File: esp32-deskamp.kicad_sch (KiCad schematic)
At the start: 29 parts, among them J1 INPUT 00, J10 ADDITIONAL GPIO, J2 INPUT 01, J3 MUTE, J4 SLEEP, J5 PRE OUT, J6 LFE OUT, J7 INPUT SELECT, J8 MOTOR, J9 12V IN, K1 INPUT 00, K2 INPUT 01, K3 AMP MUTE, K4 AMP SLEEP, U1 ESP32 D1 MINI, U2 TSR 1-2433, U3 L9110, U4 ULN2003A

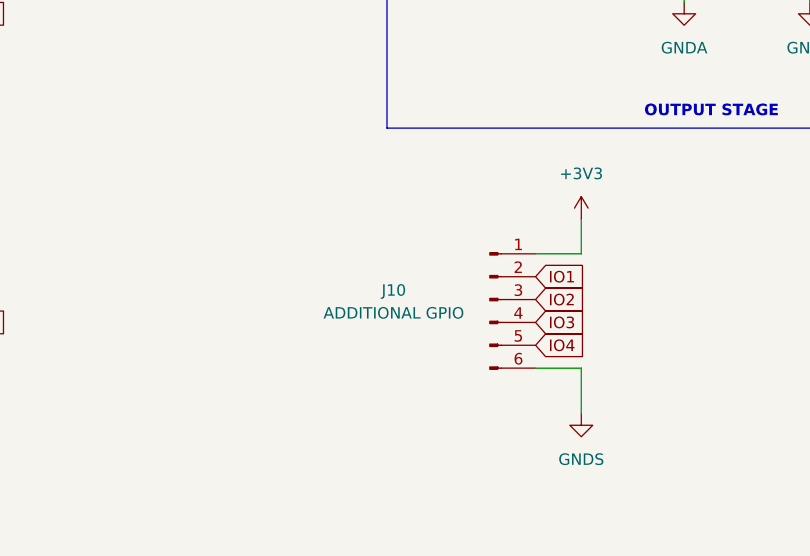
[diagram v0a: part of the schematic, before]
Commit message: Move cap
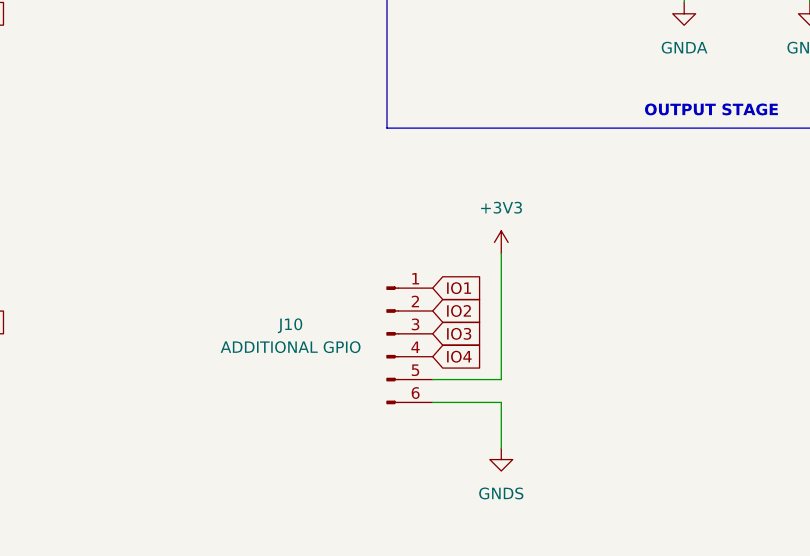
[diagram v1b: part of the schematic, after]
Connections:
- net +3V3: now also J10.5 (Pin_5); no longer J10.1 (Pin_1)
- net IO1: now also J10.1 (Pin_1); no longer J10.2 (Pin_2)
- net IO2: now also J10.2 (Pin_2); no longer J10.3 (Pin_3)
- net IO3: now also J10.3 (Pin_3); no longer J10.4 (Pin_4)
- net IO4: now also J10.4 (Pin_4); no longer J10.5 (Pin_5)
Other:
- moved on the sheet: J10
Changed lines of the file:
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@@
 	(wire
 		(pts
+			(xy 148.59 173.99) (xy 156.21 173.99)
+		)
+		(stroke
+			(width 0)
+			(type default)
+		)
+	)
+	(wire
+		(pts
 			(xy 46.99 31.75) (xy 46.99 41.91)
 		)
@@
 	(wire
 		(pts
-			(xy 165.1 172.72) (xy 165.1 177.8)
+			(xy 156.21 176.53) (xy 156.21 181.61)
 		)
 		(stroke
@@
 	(wire
 		(pts
-			(xy 160.02 160.02) (xy 165.1 160.02)
+			(xy 156.21 160.02) (xy 156.21 173.99)
 		)
 		(stroke
@@
 	(wire
 		(pts
-			(xy 160.02 172.72) (xy 165.1 172.72)
+			(xy 148.59 176.53) (xy 156.21 176.53)
 		)
 		(stroke
@@
 	(wire
 		(pts
-			(xy 165.1 156.21) (xy 165.1 160.02)
-		)
-		(stroke
-			(width 0)
-			(type default)
-		)
-	)
-	(wire
-		(pts
 			(xy 224.79 62.23) (xy 224.79 57.15)
 		)
@@
 	(global_label "IO3"
 		(shape input)
-		(at 160.02 167.64 0)
+		(at 148.59 168.91 0)
 		(fields_autoplaced yes)
 		(effects
@@
 		)
 		(property "Intersheetrefs" "${INTERSHEET_REFS}"
-			(at 166.15 167.64 0)
+			(at 154.72 168.91 0)
 			(effects
 				(font
@@
 	(global_label "IO1"
 		(shape input)
-		(at 160.02 162.56 0)
+		(at 148.59 163.83 0)
 		(fields_autoplaced yes)
 		(effects
@@
 		)
 		(property "Intersheetrefs" "${INTERSHEET_REFS}"
-			(at 166.15 162.56 0)
+			(at 154.72 163.83 0)
 			(effects
 				(font
@@
 	(global_label "IO4"
 		(shape input)
-		(at 160.02 170.18 0)
+		(at 148.59 171.45 0)
 		(fields_autoplaced yes)
 		(effects
@@
 		)
 		(property "Intersheetrefs" "${INTERSHEET_REFS}"
-			(at 166.15 170.18 0)
+			(at 154.72 171.45 0)
 			(effects
 				(font
@@
 	(global_label "IO2"
 		(shape input)
-		(at 160.02 165.1 0)
+		(at 148.59 166.37 0)
 		(fields_autoplaced yes)
 		(effects
@@
 		)
 		(property "Intersheetrefs" "${INTERSHEET_REFS}"
-			(at 166.15 165.1 0)
+			(at 154.72 166.37 0)
 			(effects
 				(font
@@
 	(symbol
 		(lib_id "power:+3V3")
-		(at 165.1 156.21 0)
+		(at 156.21 160.02 0)
 		(unit 1)
 		(exclude_from_sim no)
@@
 		(fields_autoplaced yes)
 		(property "Reference" "#PWR027"
-			(at 165.1 160.02 0)
+			(at 156.21 163.83 0)
 			(effects
 				(font
@@
 		)
 		(property "Value" "+3V3"
-			(at 165.1 151.13 0)
+			(at 156.21 154.94 0)
 			(effects
 				(font
@@
 		)
 		(property "Footprint" ""
-			(at 165.1 156.21 0)
+			(at 156.21 160.02 0)
 			(effects
 				(font
@@
 		)
 		(property "Datasheet" ""
-			(at 165.1 156.21 0)
+			(at 156.21 160.02 0)
 			(effects
 				(font
@@
 		)
 		(property "Description" "Power symbol creates a global label with name \"+3V3\""
-			(at 165.1 156.21 0)
+			(at 156.21 160.02 0)
 			(effects
 				(font
@@
 	(symbol
 		(lib_id "power:GNDS")
-		(at 165.1 177.8 0)
+		(at 156.21 181.61 0)
 		(unit 1)
 		(exclude_from_sim no)
@@
 		(fields_autoplaced yes)
 		(property "Reference" "#PWR028"
-			(at 165.1 184.15 0)
+			(at 156.21 187.96 0)
 			(effects
 				(font
@@
 		)
 		(property "Value" "GNDS"
-			(at 165.1 182.88 0)
+			(at 156.21 186.69 0)
 			(effects
 				(font
@@
 		)
 		(property "Footprint" ""
-			(at 165.1 177.8 0)
+			(at 156.21 181.61 0)
 			(effects
 				(font
@@
 		)
 		(property "Datasheet" ""
-			(at 165.1 177.8 0)
+			(at 156.21 181.61 0)
 			(effects
 				(font
@@
 		)
 		(property "Description" "Power symbol creates a global label with name \"GNDS\" , signal ground"
-			(at 165.1 177.8 0)
+			(at 156.21 181.61 0)
 			(effects
 				(font
@@
 	(symbol
 		(lib_id "Connector:Conn_01x06_Pin")
-		(at 154.94 165.1 0)
+		(at 143.51 168.91 0)
 		(unit 1)
 		(exclude_from_sim no)
@@
 		(dnp no)
 		(property "Reference" "J10"
-			(at 144.272 164.084 0)
+			(at 132.842 167.894 0)
 			(effects
 				(font
@@
 		)
 		(property "Value" "ADDITIONAL GPIO"
-			(at 144.272 166.624 0)
+			(at 132.842 170.434 0)
 			(effects
 				(font
@@
 		)
 		(property "Footprint" "Connector_PinHeader_2.54mm:PinHeader_1x06_P2.54mm_Vertical"
-			(at 154.94 165.1 0)
+			(at 143.51 168.91 0)
 			(effects
 				(font
@@
 		)
 		(property "Datasheet" "~"
-			(at 154.94 165.1 0)
+			(at 143.51 168.91 0)
 			(effects
 				(font
@@
 		)
 		(property "Description" "Generic connector, single row, 01x06, script generated"
-			(at 154.94 165.1 0)
+			(at 143.51 168.91 0)
 			(effects
 				(font
